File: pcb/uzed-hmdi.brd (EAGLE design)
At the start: 68.6 x 53 mm, 4 parts

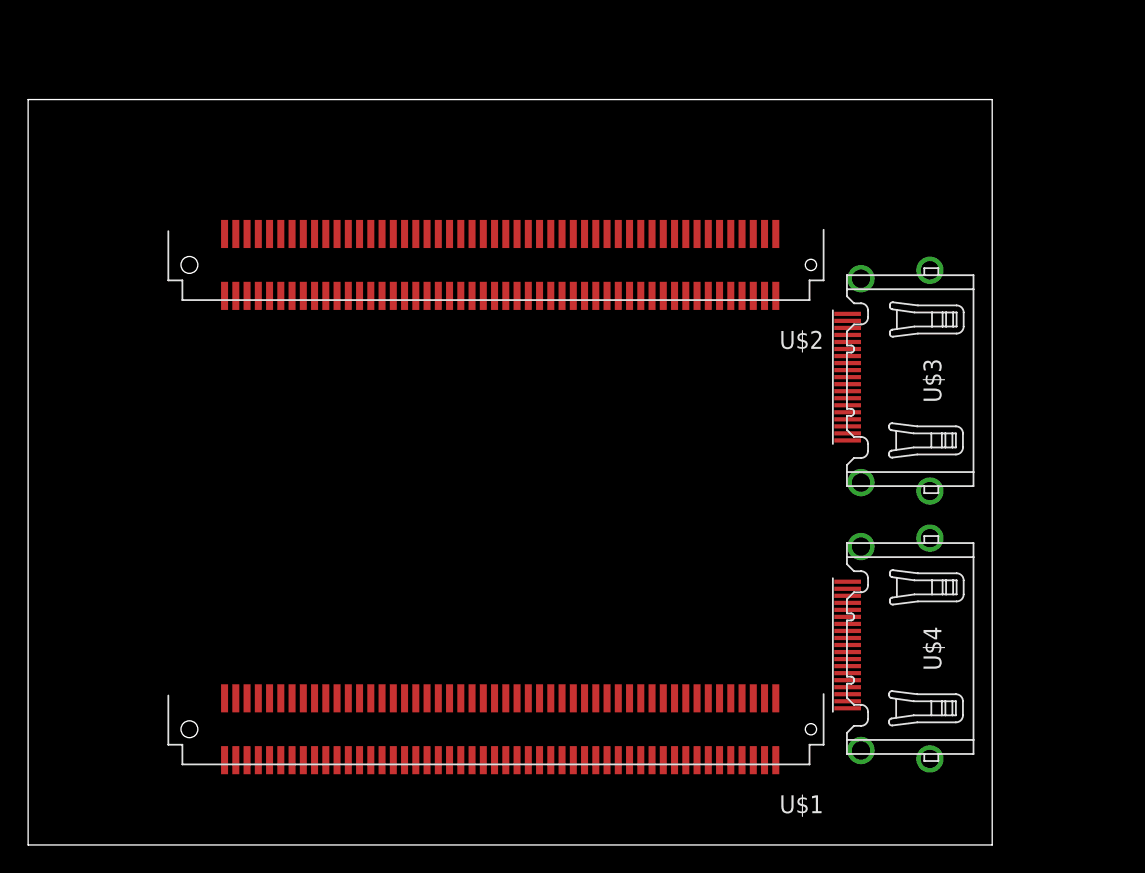
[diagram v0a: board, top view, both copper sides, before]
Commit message: prog xtal breakout and work on hdmi board
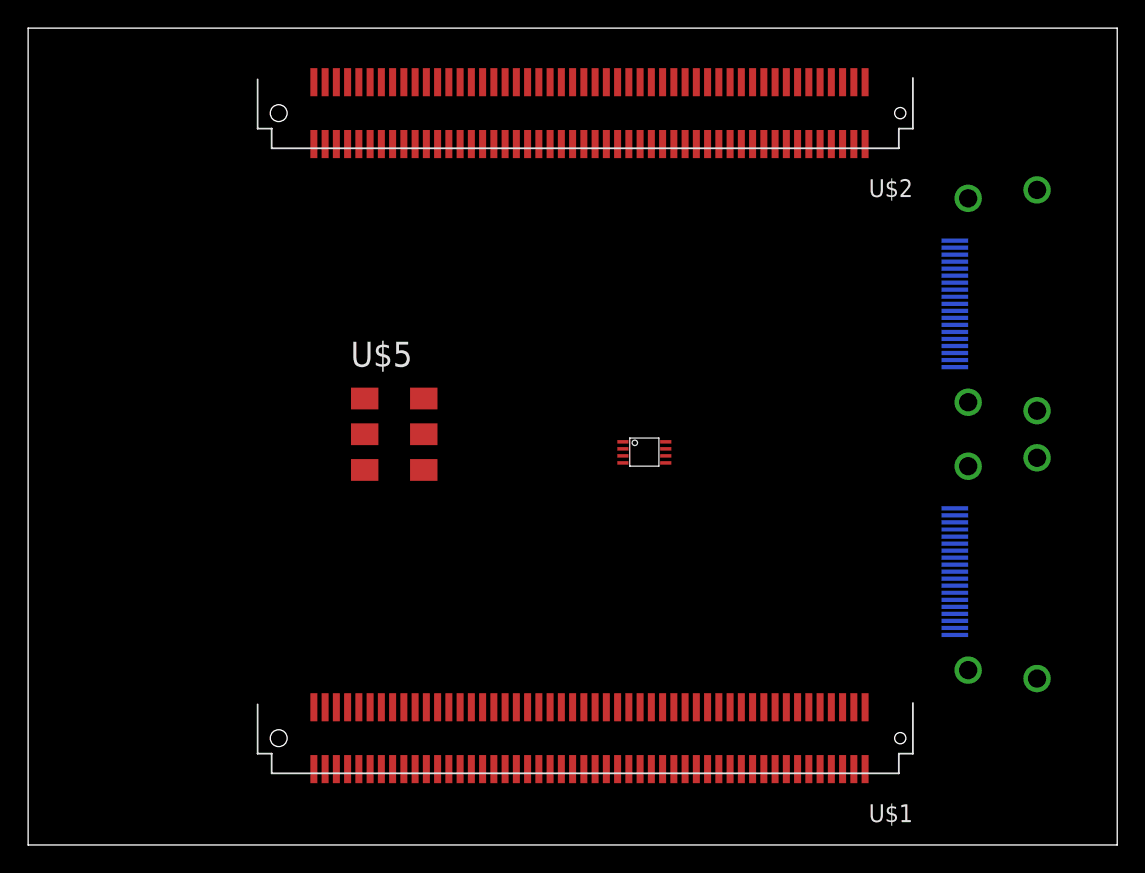
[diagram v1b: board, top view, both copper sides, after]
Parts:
- added U$5: SI514, lupa300-components:XTAL-6PIN
- added U11: PCA9306, saanlima:PSOP-8
- moved U$2 12.5 mm to (20.3, 55.2)
- moved U$4 9.52 mm to (69.8, 19.7), flipped to the bottom, turned to 270 degrees
- moved U$3 9.52 mm to (69.8, 38.7), flipped to the bottom, turned to 270 degrees
- moved U$1 6.38 mm to (20.3, 10.8)
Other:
- board size 68.6 x 53 mm -> 77.5 x 58.1 mm
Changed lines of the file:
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@@
 <setting verticaltext="up"/>
 </settings>
-<grid distance="50" unitdist="mil" unit="mil" style="lines" multiple="1" display="yes" altdistance="5" altunitdist="mil" altunit="mil"/>
+<grid distance="25" unitdist="mil" unit="mil" style="lines" multiple="1" display="yes" altdistance="5" altunitdist="mil" altunit="mil"/>
 <layers>
 <layer number="1" name="Top" color="4" fill="1" visible="yes" active="yes"/>
@@
 <layer number="108" name="tplace-old" color="10" fill="1" visible="yes" active="yes"/>
 <layer number="109" name="ref-old" color="11" fill="1" visible="yes" active="yes"/>
+<layer number="110" name="fp0" color="7" fill="1" visible="no" active="yes"/>
+<layer number="111" name="tGTest" color="7" fill="1" visible="no" active="yes"/>
+<layer number="112" name="bGTest" color="7" fill="1" visible="no" active="yes"/>
 <layer number="116" name="Patch_BOT" color="7" fill="1" visible="yes" active="yes"/>
 <layer number="121" name="_tsilk" color="7" fill="1" visible="no" active="yes"/>
 <layer number="122" name="_bsilk" color="7" fill="1" visible="no" active="yes"/>
+<layer number="123" name="tTestmark" color="7" fill="1" visible="no" active="yes"/>
+<layer number="124" name="bTestmark" color="7" fill="1" visible="no" active="yes"/>
 <layer number="125" name="_tNames" color="7" fill="1" visible="no" active="yes"/>
+<layer number="126" name="_bNames" color="5" fill="1" visible="no" active="yes"/>
+<layer number="127" name="_tValues" color="7" fill="1" visible="no" active="yes"/>
+<layer number="128" name="_bValues" color="7" fill="1" visible="no" active="yes"/>
+<layer number="131" name="prix" color="7" fill="1" visible="no" active="yes"/>
+<layer number="132" name="test" color="7" fill="1" visible="no" active="yes"/>
+<layer number="133" name="Ports" color="7" fill="1" visible="no" active="yes"/>
+<layer number="134" name="Port2" color="7" fill="1" visible="no" active="yes"/>
+<layer number="135" name="Port3" color="7" fill="1" visible="no" active="yes"/>
 <layer number="144" name="Drill_legend" color="7" fill="1" visible="no" active="yes"/>
+<layer number="150" name="Notes" color="7" fill="1" visible="no" active="yes"/>
 <layer number="151" name="HeatSink" color="7" fill="1" visible="no" active="yes"/>
+<layer number="152" name="_bDocu" color="7" fill="1" visible="no" active="yes"/>
 <layer number="199" name="Contour" color="7" fill="1" visible="yes" active="yes"/>
 <layer number="200" name="200bmp" color="1" fill="10" visible="yes" active="yes"/>
@@
 <layer number="223" name="223bmp" color="24" fill="1" visible="no" active="no"/>
 <layer number="224" name="224bmp" color="25" fill="1" visible="no" active="no"/>
+<layer number="231" name="Eagle3D_PG1" color="14" fill="1" visible="no" active="yes"/>
+<layer number="232" name="Eagle3D_PG2" color="14" fill="2" visible="no" active="yes"/>
+<layer number="233" name="Eagle3D_PG3" color="14" fill="4" visible="no" active="yes"/>
 <layer number="250" name="Descript" color="3" fill="1" visible="no" active="no"/>
 <layer number="251" name="SMDround" color="12" fill="11" visible="no" active="no"/>
 <layer number="254" name="OrgLBR" color="7" fill="1" visible="yes" active="yes"/>
+<layer number="255" name="xfer" color="7" fill="1" visible="no" active="yes"/>
 </layers>
 <board>
 <plain>
-<wire x1="0" y1="0" x2="68.56" y2="0" width="0" layer="20"/>
-<wire x1="68.56" y1="0" x2="68.56" y2="53.01" width="0" layer="20"/>
-<wire x1="68.56" y1="53.01" x2="0" y2="53.01" width="0" layer="20"/>
-<wire x1="0" y1="53.01" x2="0" y2="0" width="0" layer="20"/>
-<dimension x1="11.43" y1="7.62" x2="11.43" y2="43.18" x3="-1.27" y3="25.4" textsize="1.778" layer="1"/>
+<wire x1="0" y1="0" x2="77.45" y2="0" width="0" layer="20"/>
+<wire x1="77.45" y1="0" x2="77.45" y2="58.09" width="0" layer="20"/>
+<wire x1="77.45" y1="58.09" x2="0" y2="58.09" width="0" layer="20"/>
+<wire x1="0" y1="58.09" x2="0" y2="0" width="0" layer="20"/>
+<dimension x1="11.43" y1="7.62" x2="11.43" y2="52.07" x3="89.535" y3="29.845" textsize="1.778" layer="1" unit="mil"/>
 </plain>
 <attributes>
@@
 </autorouter>
 <elements>
-<element name="U$1" library="lupa300-components" package="BERG100POS" value="BERGSTAK-100POS" x="13.97" y="11.43" rot="R180"/>
-<element name="U$2" library="lupa300-components" package="BERG100POS" value="BERGSTAK-100POS" x="13.97" y="44.45" rot="R180"/>
-<element name="U$3" library="new-connectors" package="HDMI_A" value="HDMI-A" x="62.23" y="33.02" rot="R90"/>
-<element name="U$4" library="new-connectors" package="HDMI_A" value="HDMI-A" x="62.23" y="13.97" rot="R90"/>
+<element name="U$1" library="lupa300-components" package="BERG100POS" value="BERGSTAK-100POS" x="20.32" y="10.795" rot="R180"/>
+<element name="U$2" library="lupa300-components" package="BERG100POS" value="BERGSTAK-100POS" x="20.32" y="55.245" rot="R180"/>
+<element name="U$3" library="new-connectors" package="HDMI_A" value="HDMI-A" x="69.85" y="38.735" rot="MR270"/>
+<element name="U$4" library="new-connectors" package="HDMI_A" value="HDMI-A" x="69.85" y="19.685" rot="MR270"/>
+<element name="U$5" library="lupa300-components" package="XTAL-6PIN" value="SI514" x="26.035" y="29.21"/>
+<element name="U11" library="saanlima" package="PSOP-8" value="PCA9306" x="43.815" y="27.94" rot="R270"/>
 </elements>
 <signals>
